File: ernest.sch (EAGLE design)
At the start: 26 parts, among them IC1 ATMEGA328-P, SW1 IDENT, Y1 16MHz

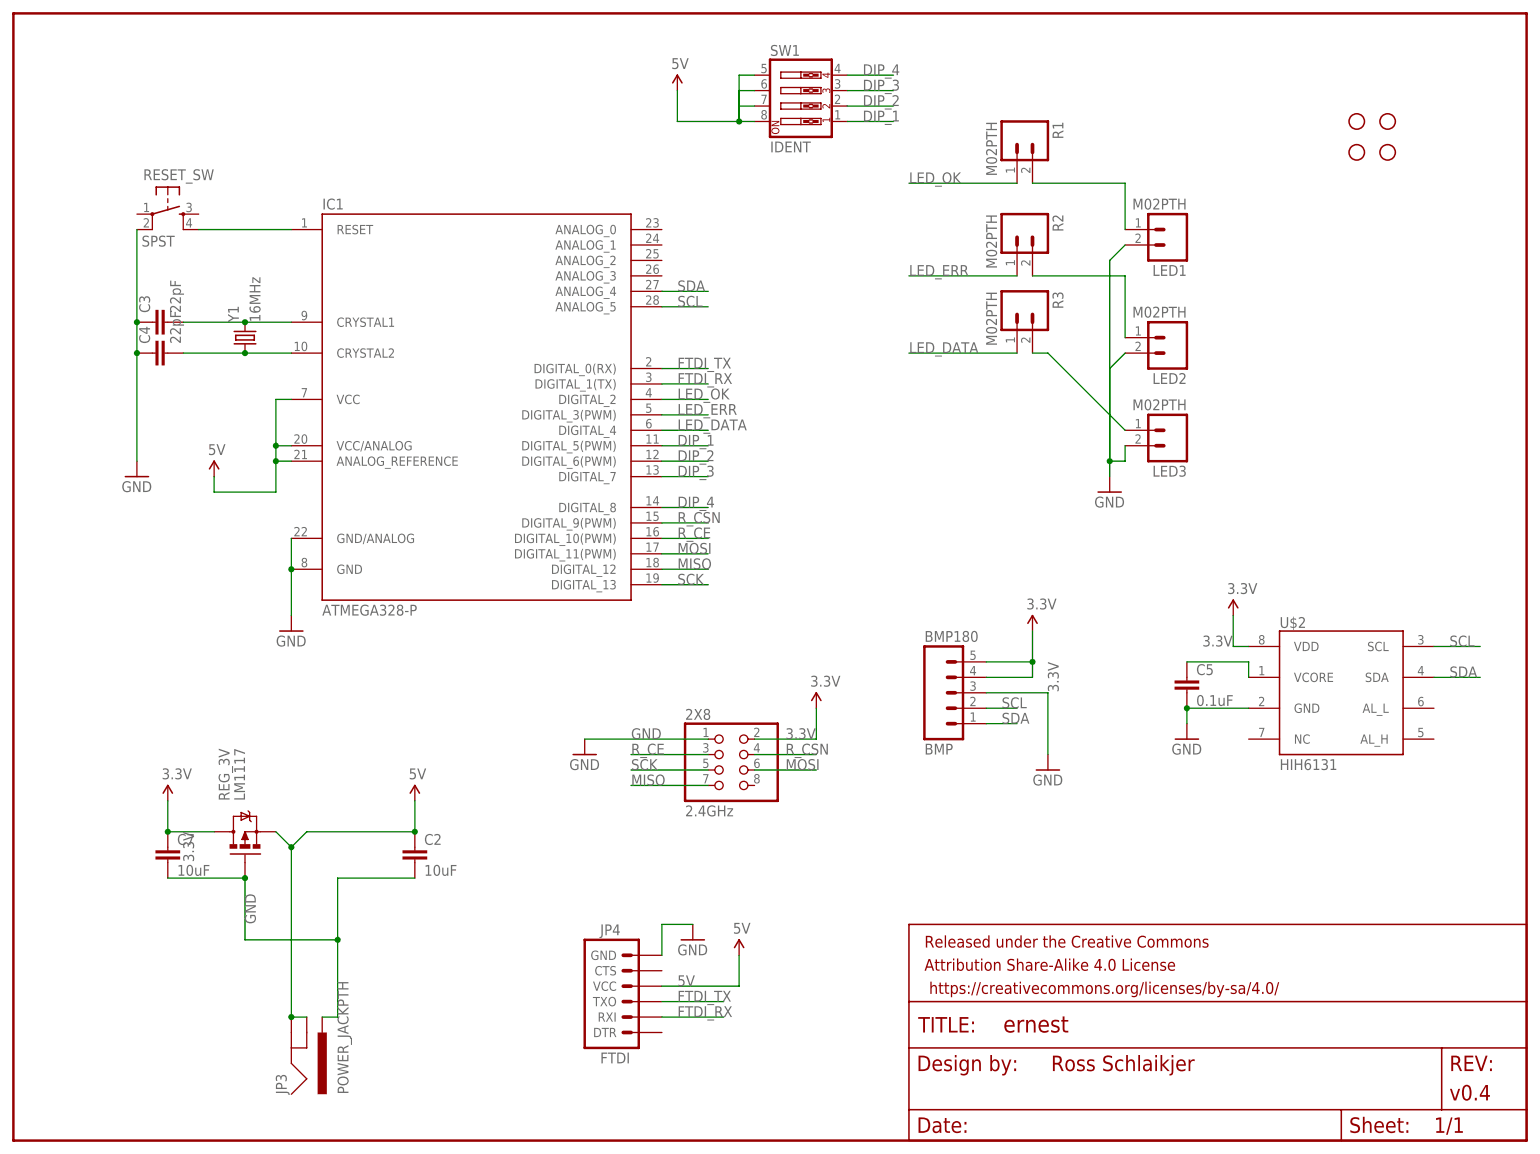
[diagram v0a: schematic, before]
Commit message: V0.4 release
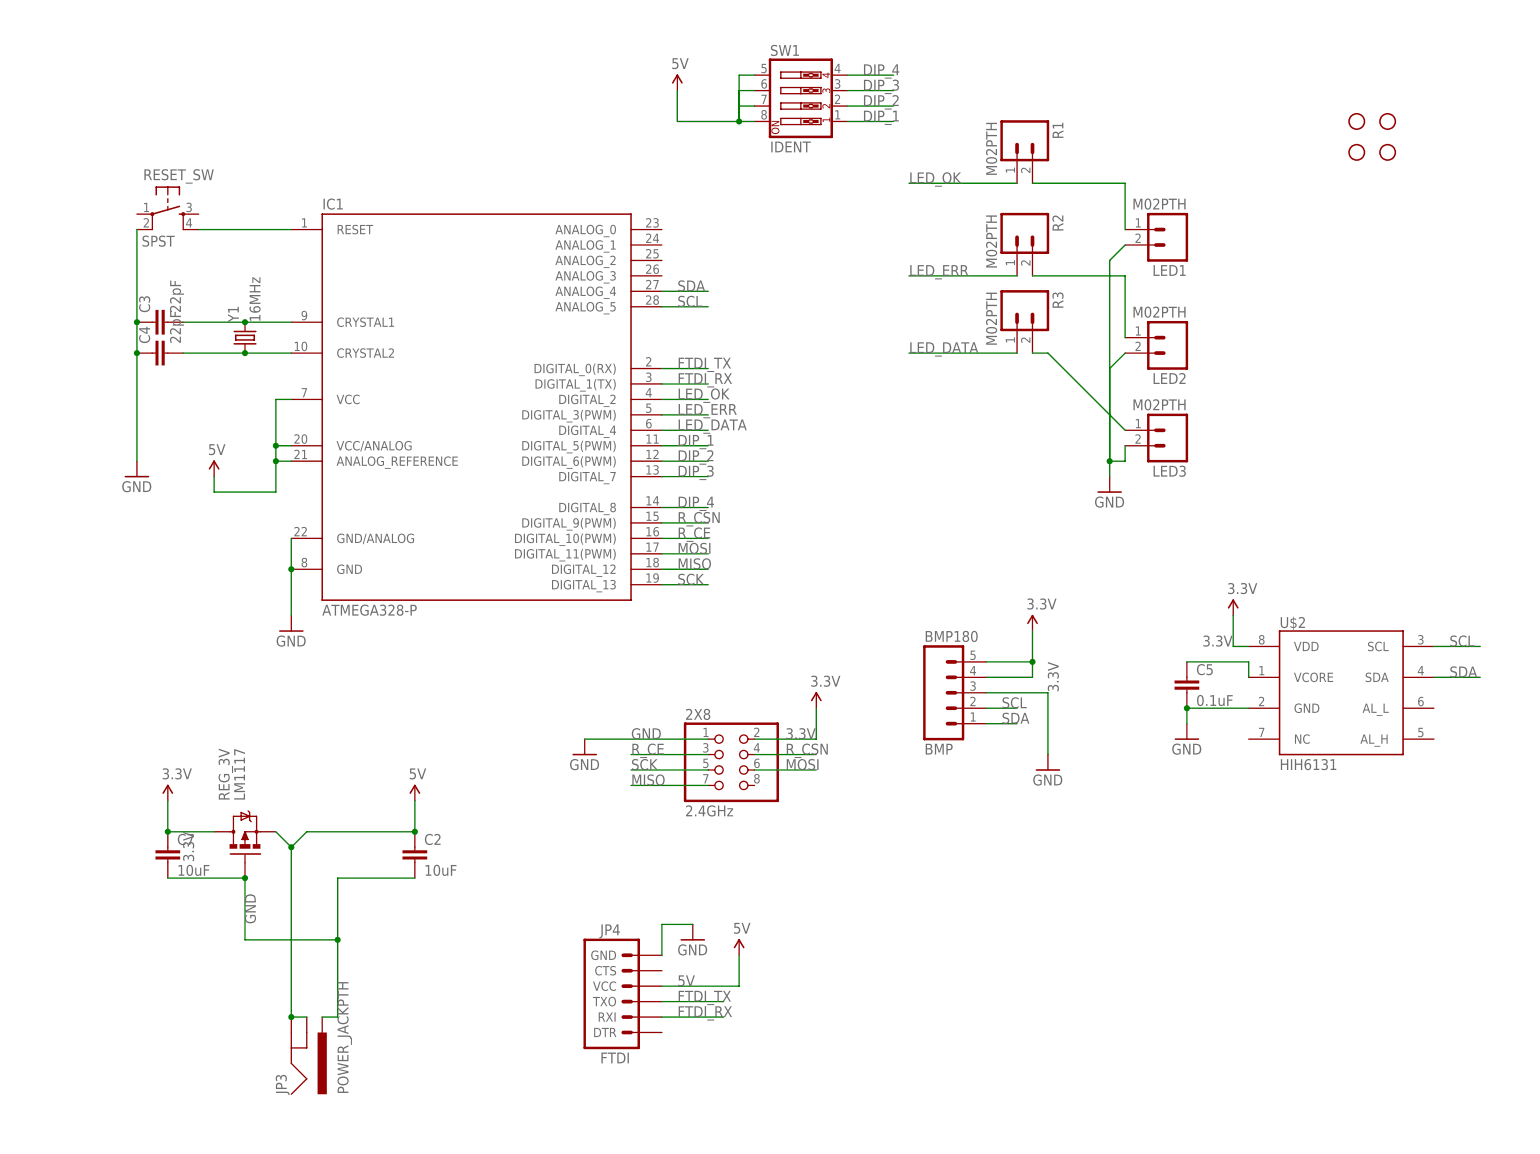
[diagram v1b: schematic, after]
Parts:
- removed ERNEST: Ernest, SparkFun-Aesthetics:FRAME-LETTER
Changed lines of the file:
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@@
 <part name="REG_3V" library="User-Submitted" deviceset="MOSFET-PCHANNEL" device="FQP27P06" value="LM1117"/>
 <part name="BMP180" library="SparkFun-Connectors" deviceset="M05" device="PTH" value="BMP"/>
-<part name="ERNEST" library="SparkFun-Aesthetics" deviceset="FRAME-LETTER" device="" value="Ernest">
-<attribute name="DESIGNER" value="Ross Schlaikjer"/>
-<attribute name="VERSION" value="v0.4"/>
-</part>
 <part name="JP4" library="SparkFun-Connectors" deviceset="ARDUINO_SERIAL_PROGRAM" device="PTH" value="FTDI"/>
 <part name="SUPPLY1" library="SparkFun-Aesthetics" deviceset="3.3V" device=""/>
@@
 <instance part="REG_3V" gate="G$1" x="-121.92" y="-20.32" rot="R90"/>
 <instance part="BMP180" gate="G$1" x="-7.62" y="2.54"/>
-<instance part="ERNEST" gate="G$1" x="-160.02" y="-71.12"/>
-<instance part="ERNEST" gate="V" x="-12.7" y="-71.12"/>
 <instance part="JP4" gate="G$1" x="-58.42" y="-48.26"/>
 <instance part="SUPPLY1" gate="G$1" x="7.62" y="12.7"/>
